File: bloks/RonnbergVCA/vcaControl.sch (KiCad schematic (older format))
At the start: 14 parts, among them J1C1 Conn_01x01, J2C1 Conn_01x01, J3C1 Conn_01x01, J4C1 Conn_01x01, J5C1 Conn_01x01, J6C1 Conn_01x01

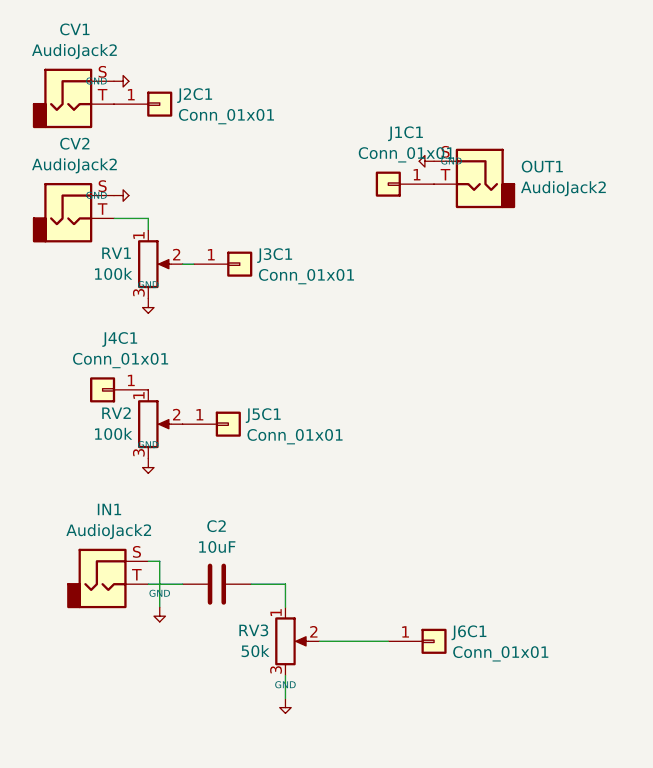
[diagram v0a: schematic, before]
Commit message: pcb layout
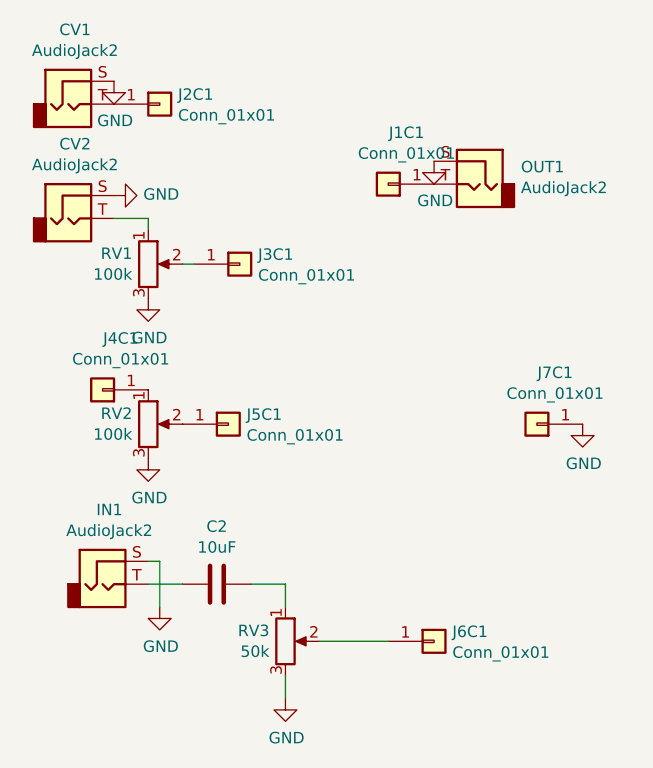
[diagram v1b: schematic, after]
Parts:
- added J7C1: Conn_01x01, Connector_PinHeader_2.54mm:PinHeader_1x01_P2.54mm_Vertical, symbol Connector_Generic:Conn_01x01
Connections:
- net +5V renamed GND
- net GND: now also J7C1.1 (Pin_1)
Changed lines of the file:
@@
 Wire Wire Line
 	9050 3350 9350 3350
-$Comp
-L keyboard_parts:GND #PWR0102
-U 1 1 5CB3B890
-P 8300 2550
-F 0 "#PWR0102" H 8300 2600 20  0001 C CNN
-F 1 "GND" H 8300 2609 30  0000 C CNN
-F 2 "" H 8300 2550 60  0000 C CNN
-F 3 "" H 8300 2550 60  0000 C CNN
-	1    8300 2550
-	1    0    0    -1
-$EndComp
-$Comp
-L keyboard_parts:GND #PWR0103
-U 1 1 5CB3B8CE
-P 8300 1850
-F 0 "#PWR0103" H 8300 1900 20  0001 C CNN
-F 1 "GND" H 8300 1909 30  0000 C CNN
-F 2 "" H 8300 1850 60  0000 C CNN
-F 3 "" H 8300 1850 60  0000 C CNN
-	1    8300 1850
-	1    0    0    -1
-$EndComp
-$Comp
-L keyboard_parts:GND #PWR0105
-U 1 1 5CB3BB4D
-P 8900 3600
-F 0 "#PWR0105" H 8900 3650 20  0001 C CNN
-F 1 "GND" H 8900 3659 30  0000 C CNN
-F 2 "" H 8900 3600 60  0000 C CNN
-F 3 "" H 8900 3600 60  0000 C CNN
-	1    8900 3600
-	1    0    0    -1
-$EndComp
 Wire Wire Line
 	8900 3500 8900 3600
@@
 Wire Wire Line
 	8300 3100 8450 3100
-$Comp
-L keyboard_parts:GND #PWR0111
-U 1 1 5CB452C5
-P 8350 3200
-F 0 "#PWR0111" H 8350 3250 20  0001 C CNN
-F 1 "GND" H 8350 3259 30  0000 C CNN
-F 2 "" H 8350 3200 60  0000 C CNN
-F 3 "" H 8350 3200 60  0000 C CNN
-	1    8350 3200
-	1    0    0    -1
-$EndComp
 Wire Wire Line
 	8350 3200 8350 3000
@@
 $EndComp
 $Comp
-L keyboard_parts:GND #PWR?
-U 1 1 5CC61B5F
+L power:GND #PWR?
+U 1 1 5CC8FB4A
 P 8150 900
-F 0 "#PWR?" H 8150 950 20  0001 C CNN
-F 1 "GND" V 8150 929 30  0000 L CNN
-F 2 "" H 8150 900 60  0000 C CNN
-F 3 "" H 8150 900 60  0000 C CNN
+F 0 "#PWR?" H 8150 650 50  0001 C CNN
+F 1 "GND" H 8155 727 50  0000 C CNN
+F 2 "" H 8150 900 50  0001 C CNN
+F 3 "" H 8150 900 50  0001 C CNN
 	1    8150 900
-	0    -1   -1   0
-$EndComp
-$Comp
-L keyboard_parts:GND #PWR?
-U 1 1 5CC61BC7
+	1    0    0    -1
+$EndComp
+$Comp
+L power:GND #PWR?
+U 1 1 5CC8FB88
 P 8150 1400
-F 0 "#PWR?" H 8150 1450 20  0001 C CNN
-F 1 "GND" V 8150 1429 30  0000 L CNN
-F 2 "" H 8150 1400 60  0000 C CNN
-F 3 "" H 8150 1400 60  0000 C CNN
+F 0 "#PWR?" H 8150 1150 50  0001 C CNN
+F 1 "GND" V 8155 1272 50  0000 R CNN
+F 2 "" H 8150 1400 50  0001 C CNN
+F 3 "" H 8150 1400 50  0001 C CNN
 	1    8150 1400
 	0    -1   -1   0
 $EndComp
 $Comp
-L keyboard_parts:GND #PWR?
-U 1 1 5CC61C2F
+L power:GND #PWR?
+U 1 1 5CC8FBF0
+P 8300 2550
+F 0 "#PWR?" H 8300 2300 50  0001 C CNN
+F 1 "GND" H 8305 2377 50  0000 C CNN
+F 2 "" H 8300 2550 50  0001 C CNN
+F 3 "" H 8300 2550 50  0001 C CNN
+	1    8300 2550
+	1    0    0    -1
+$EndComp
+$Comp
+L power:GND #PWR?
+U 1 1 5CC8FC2E
+P 8350 3200
+F 0 "#PWR?" H 8350 2950 50  0001 C CNN
+F 1 "GND" H 8355 3027 50  0000 C CNN
+F 2 "" H 8350 3200 50  0001 C CNN
+F 3 "" H 8350 3200 50  0001 C CNN
+	1    8350 3200
+	1    0    0    -1
+$EndComp
+$Comp
+L power:GND #PWR?
+U 1 1 5CC8FC6C
+P 8300 1850
+F 0 "#PWR?" H 8300 1600 50  0001 C CNN
+F 1 "GND" H 8305 1677 50  0000 C CNN
+F 2 "" H 8300 1850 50  0001 C CNN
+F 3 "" H 8300 1850 50  0001 C CNN
+	1    8300 1850
+	1    0    0    -1
+$EndComp
+$Comp
+L power:GND #PWR?
+U 1 1 5CC8FCE2
+P 8900 3600
+F 0 "#PWR?" H 8900 3350 50  0001 C CNN
+F 1 "GND" H 8905 3427 50  0000 C CNN
+F 2 "" H 8900 3600 50  0001 C CNN
+F 3 "" H 8900 3600 50  0001 C CNN
+	1    8900 3600
+	1    0    0    -1
+$EndComp
+$Comp
+L power:GND #PWR?
+U 1 1 5CC8FD2E
 P 9550 1250
-F 0 "#PWR?" H 9550 1300 20  0001 C CNN
-F 1 "GND" V 9550 1279 30  0000 L CNN
-F 2 "" H 9550 1250 60  0000 C CNN
-F 3 "" H 9550 1250 60  0000 C CNN
+F 0 "#PWR?" H 9550 1000 50  0001 C CNN
+F 1 "GND" H 9555 1077 50  0000 C CNN
+F 2 "" H 9550 1250 50  0001 C CNN
+F 3 "" H 9550 1250 50  0001 C CNN
 	1    9550 1250
-	0    1    1    0
+	1    0    0    -1
+$EndComp
+$Comp
+L power:GND #PWR?
+U 1 1 5CC8FD6C
+P 10200 2400
+F 0 "#PWR?" H 10200 2150 50  0001 C CNN
+F 1 "GND" H 10205 2227 50  0000 C CNN
+F 2 "" H 10200 2400 50  0001 C CNN
+F 3 "" H 10200 2400 50  0001 C CNN
+	1    10200 2400
+	1    0    0    -1
+$EndComp
+$Comp
+L Connector_Generic:Conn_01x01 J7C1
+U 1 1 5CC8FF50
+P 10000 2400
+F 0 "J7C1" H 9920 2175 50  0000 C CNN
+F 1 "Conn_01x01" H 9920 2266 50  0000 C CNN
+F 2 "Connector_PinHeader_2.54mm:PinHeader_1x01_P2.54mm_Vertical" H 10000 2400 50  0001 C CNN
+F 3 "~" H 10000 2400 50  0001 C CNN
+	1    10000 2400
+	-1   0    0    1
 $EndComp
 $EndSCHEMATC
